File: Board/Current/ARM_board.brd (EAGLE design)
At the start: 101.6 x 81.3 mm, 177 parts, among them IC3 STM32F437VI, IC4 LM358DT, J1 USART/I2C, J10 ANALOG, J11 DGND, J12 DPWR, J13 DIGITAL, J14 SGND, J15 SPWR, J16 SERVO, J2 I2C2/USART3, J3 USART2, J5 SPI, J6 Bluesmirf, J7 SWD, J8 AGND, J9 APWR, Q1 STL4P2UH7, Q2 2STR1230, Q3 STL4P2UH7, SW1 SW, U1 LSM330, U10 BAV99, U11 BAV99, U12 USBLC6-2, U13 USBLC6-2, U14 STMPS2171MTR, U15 MC74HC164, U3 NC7SZU04, U4 L6206Q, U5 L6206Q, U6 SI7617, U7 SI7617, U8 SI7617, U9 SI7617, Y2 8MHz

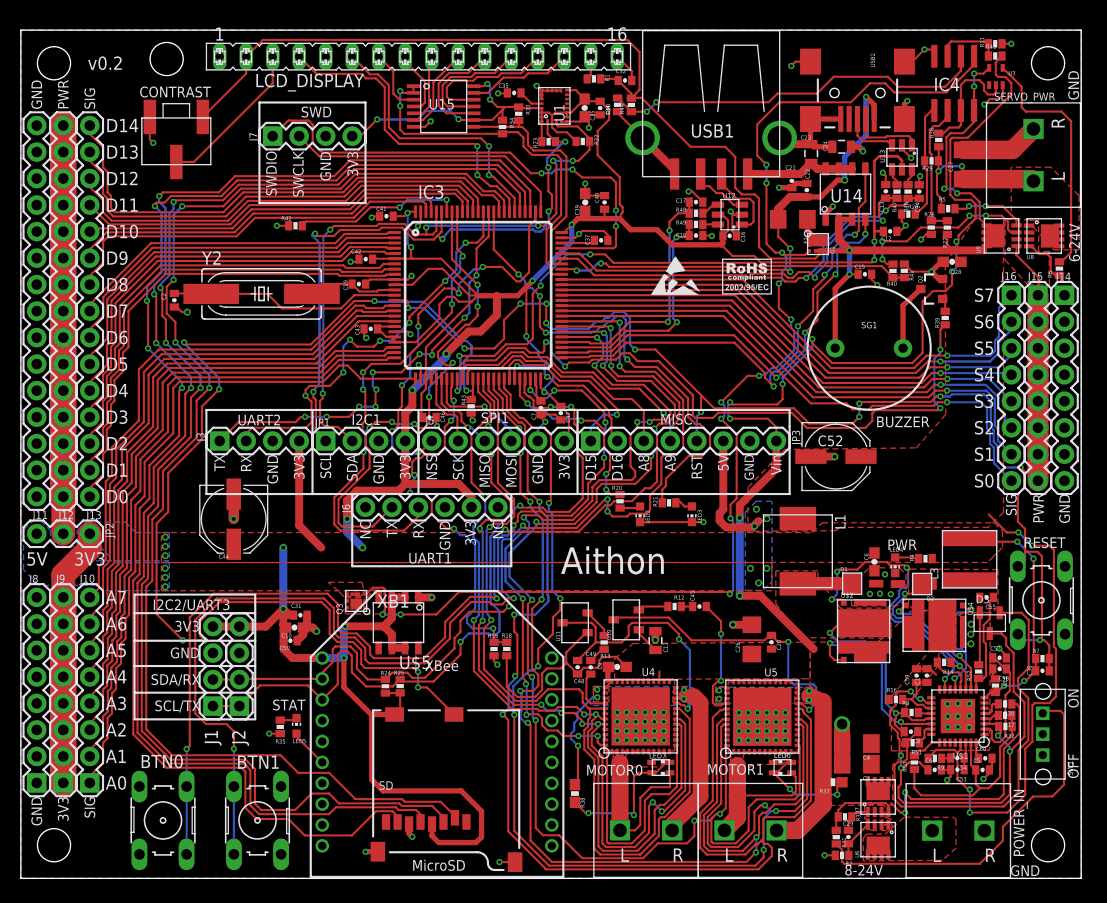
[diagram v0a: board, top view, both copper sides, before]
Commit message: Cleaned up the layout.
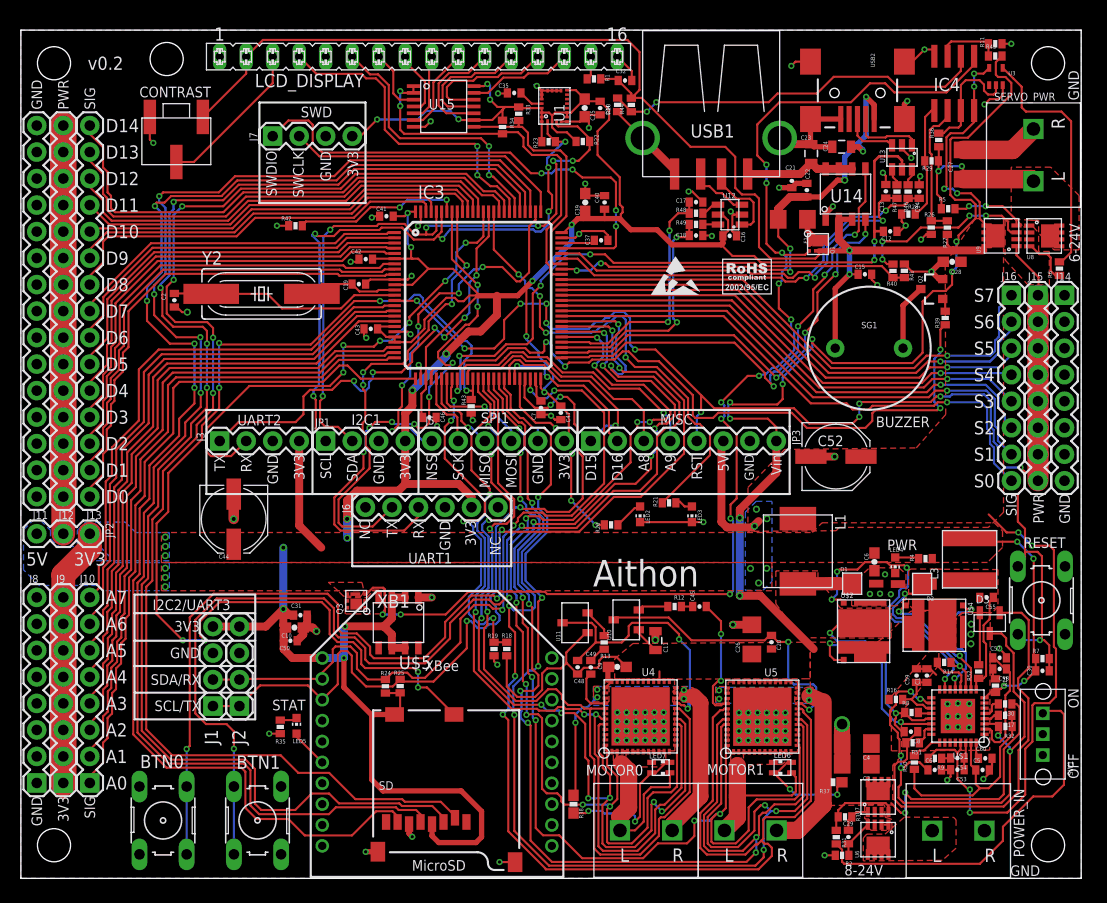
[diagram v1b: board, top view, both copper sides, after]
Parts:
- moved R20 2.42 mm to (56.6, 33.9), turned to 180 degrees
- moved R38 1.03 mm to (53.0, 7.11)
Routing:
- net M0_B: track 79.2 -> 87.3 mm
- net +3V3: track 378.9 -> 372.1 mm
- net USART2_RX: track 39.6 -> 46.3 mm, vias 7 -> 6
- net BOOT1: track 108.6 -> 104.5 mm
- net M0_FAULT: track 93.3 -> 97.3 mm
- net SPI3_MISO: track 128.0 -> 130.4 mm
- net BTN1: track 118.4 -> 116.1 mm, vias 7 -> 5
- net SPI3_MOSI: track 128.4 -> 130.5 mm
- net SPI3_SCK: track 129.6 -> 131.7 mm
- net SPI3_NSS: track 122.4 -> 124.5 mm
- net SPI1_NSS: track 38.7 -> 36.7 mm, vias 6 -> 5
- net BAT_SENSE: track 36.2 -> 34.3 mm, vias 6 -> 4
- net GND: track 152.5 -> 150.6 mm
- net I2C2_SCL/USART3_TX: track 74.5 -> 76.2 mm
- net M1_EN: track 116.8 -> 118.3 mm
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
